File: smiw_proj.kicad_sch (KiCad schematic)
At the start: 24 parts, among them J1 Conn_02x06_Odd_Even, J2 Conn_02x05_Odd_Even, J3 Conn_01x02, J4 Conn_01x02, SW1 SW_Push, U1 LM2596S-5, U2 M5 Stamp-S3, U3 LD1117S33TR_SOT223

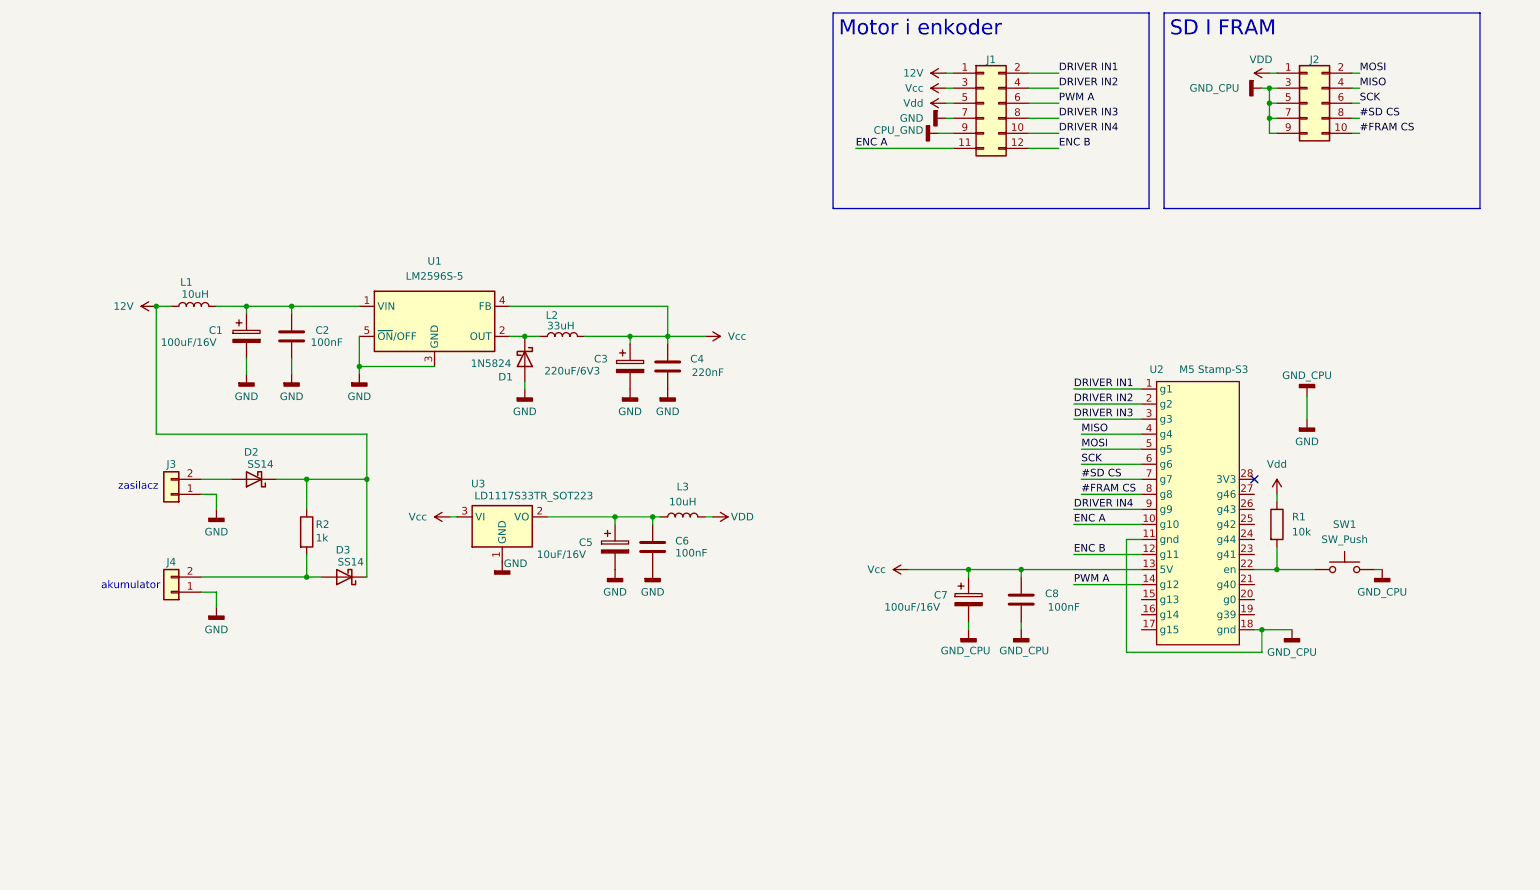
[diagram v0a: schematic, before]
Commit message: Skończone ale można zbierać informacje o dalszych szczegółach
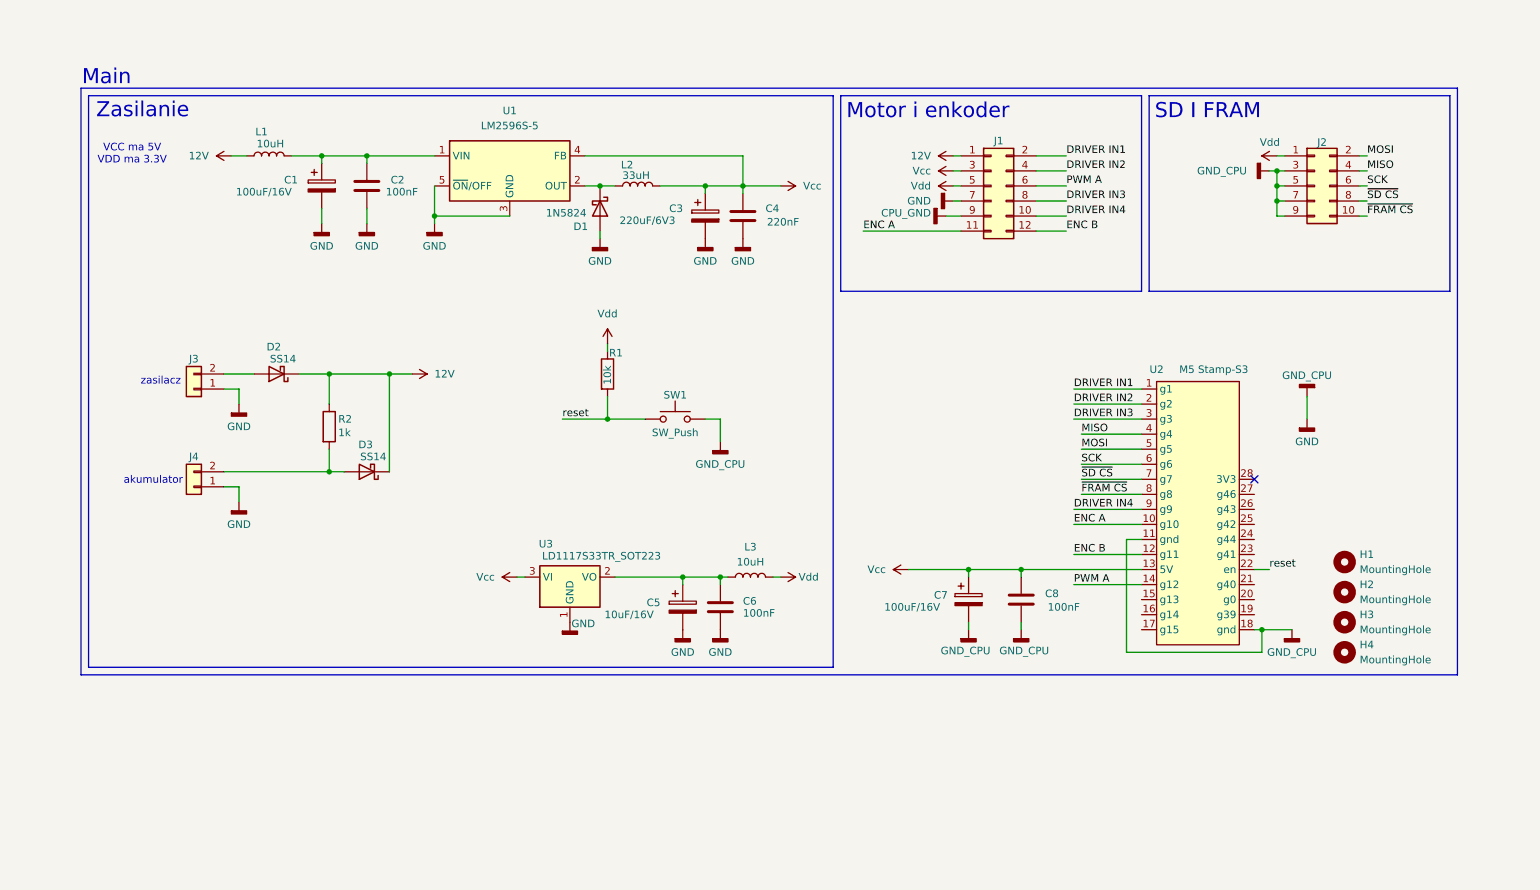
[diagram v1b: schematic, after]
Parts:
- added H1, H2, H3, H4: MountingHole, MountingHole:MountingHole_3.2mm_M3_DIN965_Pad_TopBottom, symbol Mechanical:MountingHole
- C1, C3, C5, C7: footprint (none) -> Capacitor_SMD:CP_Elec_6.3x5.3; KiLib_Generator (none) -> capacitor/THT/other
- C2, C6, C8: footprint (none) -> Capacitor_SMD:C_0805_2012Metric_Pad1.18x1.45mm_HandSolder; KiLib_Generator (none) -> SMD_2terminal_chip_molded
- C4: footprint (none) -> Capacitor_SMD:C_0805_2012Metric_Pad1.18x1.45mm_HandSolder; KiLib_Generator (none) -> capacitor/THT/other
- D1: footprint Diode_THT:D_DO-201AD_P15.24mm_Horizontal -> Diode_SMD:D_SMC; KiLib_Generator (none) -> diode/THT
- D2: footprint (none) -> Diode_SMD:D_SMC
- D3: footprint (none) -> Diode_SMD:D_SMA
- J1: footprint (none) -> Connector_PinHeader_2.54mm:PinHeader_2x06_P2.54mm_Vertical; KiLib_Generator (none) -> connector/pin_header_socket
- J2: footprint (none) -> Connector_PinSocket_1.00mm:PinSocket_2x05_P1.00mm_Vertical_SMD; KiLib_Generator (none) -> connector/pin_header_socket
- J3, J4: footprint (none) -> Connector_PinSocket_1.00mm:PinSocket_1x02_P1.00mm_Vertical_SMD_Pin1Left; KiLib_Generator (none) -> connector/pin_header_socket
- L1, L2, L3: footprint (none) -> Inductor_SMD:L_Bourns_SRR1260; KiLib_Generator (none) -> SMD_2terminal_chip_molded
- R1, R2: footprint (none) -> Resistor_SMD:R_1206_3216Metric_Pad1.30x1.75mm_HandSolder; KiLib_Generator (none) -> SMD_2terminal_chip_molded
- SW1: footprint (none) -> Button_Switch_SMD:SW_SPST_PTS647_Sx50
- U1: KiLib_Generator (none) -> package/TO_SOT/SMD
- U2: footprint stamps3254:Stamp-S3_PIN2.54_DIP -> Library2:Stamp-S3_PIN1.27_Socket
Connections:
- net VDD is gone; now on net Vdd: J2.1 (Pin_1), L3.2
- net reset: now reaches R1.2, SW1.1, U2.22 (en)
- net #FRAM CS renamed ~{FRAM CS}
- net #SD CS renamed ~{SD CS}
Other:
- note added: "Main"
- note added: "VCC ma 5V VDD ma 3.3V"
- note added: "Zasilanie"
- moved on the sheet: C1, C2, C3, C4, C5, C6, D1, D2, D3, J3, J4, L1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

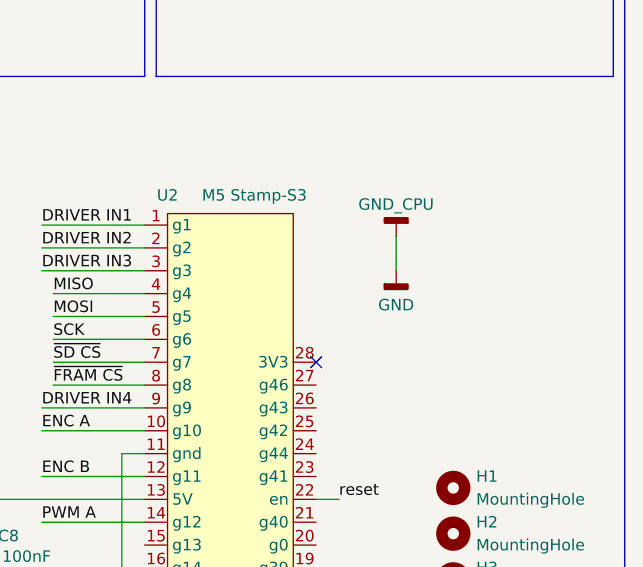
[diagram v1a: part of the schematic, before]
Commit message: rezystor
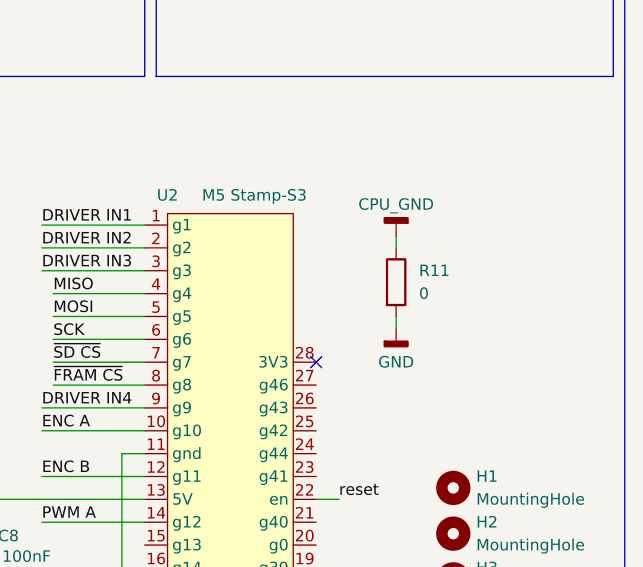
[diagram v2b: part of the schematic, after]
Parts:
- added R11: 0, Resistor_SMD:R_0805_2012Metric, symbol Device:R
- J2: footprint Connector_PinSocket_1.00mm:PinSocket_2x05_P1.00mm_Vertical_SMD -> Connector_PinSocket_2.54mm:PinSocket_2x05_P2.54mm_Vertical_SMD
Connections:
- net CPU_GND: now also R11.1
- net GND: now also R11.2; no longer C7.2, C8.1, J2.3 (Pin_3), J2.5 (Pin_5), J2.7 (Pin_7), J2.9 (Pin_9), SW1.2, U2.11 (gnd), U2.18 (gnd)
- new net GND_CPU: C7.2, C8.1, J2.3 (Pin_3), J2.5 (Pin_5), J2.7 (Pin_7), J2.9 (Pin_9), SW1.2, U2.11 (gnd), U2.18 (gnd)
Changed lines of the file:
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@@
 	(wire
 		(pts
-			(xy 240.03 86.36) (xy 240.03 82.55)
-		)
-		(stroke
-			(width 0)
-			(type default)
-		)
-	)
-	(wire
-		(pts
 			(xy 201.93 88.9) (xy 212.09 88.9)
 		)
@@
 	(wire
 		(pts
+			(xy 240.03 91.44) (xy 240.03 92.71)
+		)
+		(stroke
+			(width 0)
+			(type default)
+		)
+	)
+	(wire
+		(pts
 			(xy 69.85 78.74) (xy 74.93 78.74)
 		)
@@
 	(wire
 		(pts
+			(xy 240.03 82.55) (xy 240.03 83.82)
+		)
+		(stroke
+			(width 0)
+			(type default)
+		)
+	)
+	(wire
+		(pts
 			(xy 144.78 46.99) (xy 144.78 48.26)
 		)
@@
 			)
 		)
-		(property "Value" "GND_CPU"
+		(property "Value" "CPU_GND"
 			(at 240.03 78.994 0)
 			(show_name no)
@@
 			)
 		)
-		(property "Footprint" "Connector_PinSocket_1.00mm:PinSocket_2x05_P1.00mm_Vertical_SMD"
+		(property "Footprint" "Connector_PinSocket_2.54mm:PinSocket_2x05_P2.54mm_Vertical_SMD"
 			(at 241.3 46.99 0)
 			(hide yes)
@@
 	(symbol
 		(lib_id "power:GNDD")
-		(at 240.03 86.36 0)
+		(at 240.03 92.71 0)
 		(unit 1)
 		(body_style 1)
@@
 		(fields_autoplaced yes)
 		(property "Reference" "#PWR017"
-			(at 240.03 92.71 0)
+			(at 240.03 99.06 0)
 			(hide yes)
 			(show_name no)
@@
 		)
 		(property "Value" "GND"
-			(at 240.03 90.17 0)
+			(at 240.03 96.52 0)
 			(show_name no)
 			(do_not_autoplace no)
@@
 		)
 		(property "Footprint" ""
-			(at 240.03 86.36 0)
+			(at 240.03 92.71 0)
 			(hide yes)
 			(show_name no)
@@
 		)
 		(property "Datasheet" ""
-			(at 240.03 86.36 0)
+			(at 240.03 92.71 0)
 			(hide yes)
 			(show_name no)
@@
 		)
 		(property "Description" "Power symbol creates a global label with name \"GNDD\" , digital ground"
-			(at 240.03 86.36 0)
+			(at 240.03 92.71 0)
 			(hide yes)
 			(show_name no)
@@
 					(unit 1)
 				)
+			)
+		)
+	)
+	(symbol
+		(lib_id "Device:R")
+		(at 240.03 87.63 0)
+		(unit 1)
+		(body_style 1)
+		(exclude_from_sim no)
+		(in_bom yes)
+		(on_board yes)
+		(in_pos_files yes)
+		(dnp no)
+		(fields_autoplaced yes)
+		(property "Reference" "R11"
+			(at 242.57 86.3599 0)
+			(show_name no)
+			(do_not_autoplace no)
+			(effects
+				(font
+					(size 1.27 1.27)
+				)
+				(justify left)
+			)
+		)
+		(property "Value" "0"
+			(at 242.57 88.8999 0)
+			(show_name no)
+			(do_not_autoplace no)
+			(effects
+				(font
+					(size 1.27 1.27)
+				)
+				(justify left)
+			)
+		)
+		(property "Footprint" "Resistor_SMD:R_0805_2012Metric"
+			(at 238.252 87.63 90)
+			(hide yes)
+			(show_name no)
+			(do_not_autoplace no)
+			(effects
+				(font
+					(size 1.27 1.27)
+				)
+			)
+		)
+		(property "Datasheet" ""
+			(at 240.03 87.63 0)
+			(hide yes)
+			(show_name no)
+			(do_not_autoplace no)
+			(effects
+				(font
+					(size 1.27 1.27)
+				)
+			)
+		)
+		(property "Description" "Resistor"
+			(at 240.03 87.63 0)
+			(hide yes)
+			(show_name no)
+			(do_not_autoplace no)
+			(effects
+				(font
+					(size 1.27 1.27)
+				)
+			)
+		)
+		(pin "2"
+		)
+		(pin "1"
+		)
+		(instances
+			(project "smiw_proj"
+				(path "/8fb2202e-c9a0-482b-8823-f82b9d12ce5a"
+					(reference "R11")
+					(unit 1)
+				)

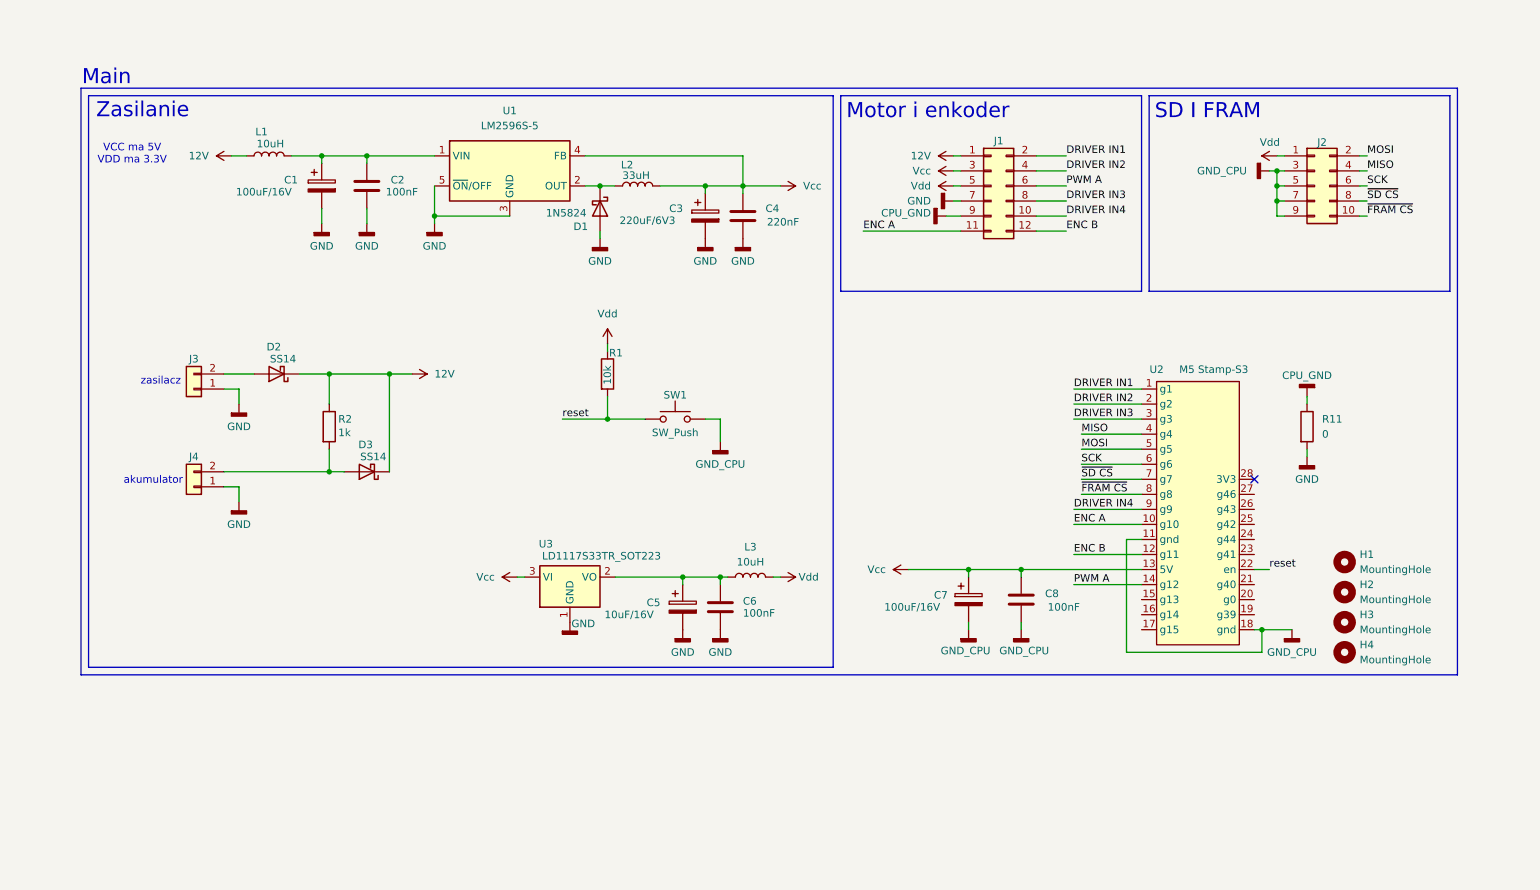
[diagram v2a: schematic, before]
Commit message: Niedziela
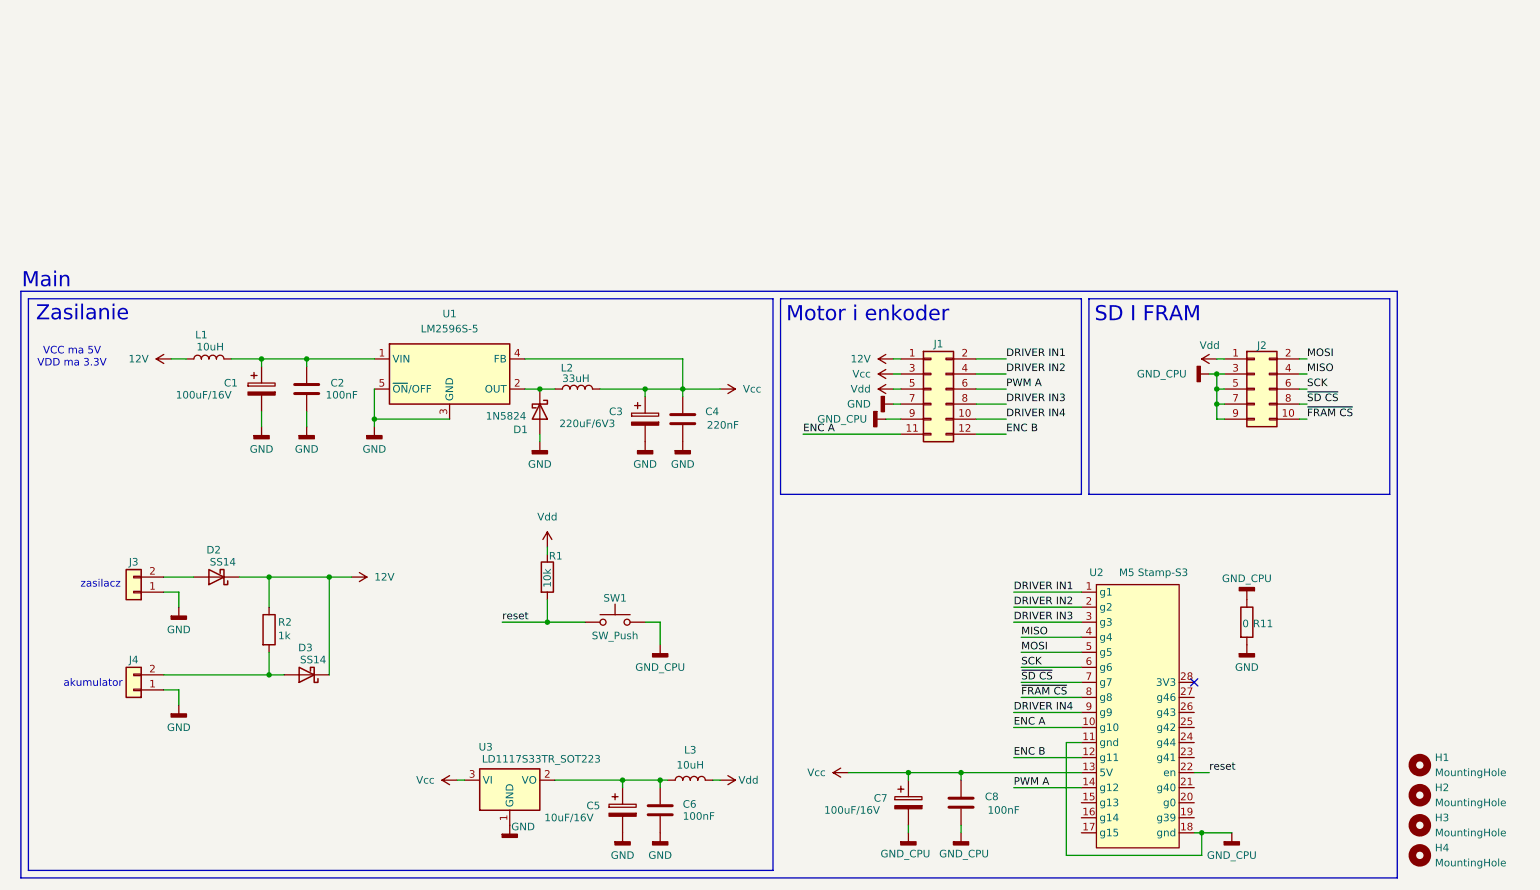
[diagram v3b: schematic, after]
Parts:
- H1, H2, H3, H4: KiLib_Generator (none) -> mounting_hardware/mounting_hole
- R11: footprint Resistor_SMD:R_0805_2012Metric -> Resistor_SMD:R_1206_3216Metric_Pad1.30x1.75mm_HandSolder; KiLib_Generator (none) -> SMD_2terminal_chip_molded
- U2: footprint Library2:Stamp-S3_PIN1.27_Socket -> Library:M5Stamp-S3
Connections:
- net CPU_GND is gone; now on net GND_CPU: J1.9 (Pin_9), R11.1
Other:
- moved on the sheet: C1, C2, C3, C4, C5, C6, C7, C8, D1, D2, D3, H1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
